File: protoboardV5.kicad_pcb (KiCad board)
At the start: 2 copper layers, 33 x 25 mm, 19 parts, among them J1 J1, J2 J2, J3 J3, M1 M1, Q1 Q1, Q2 Q2, U1 U1

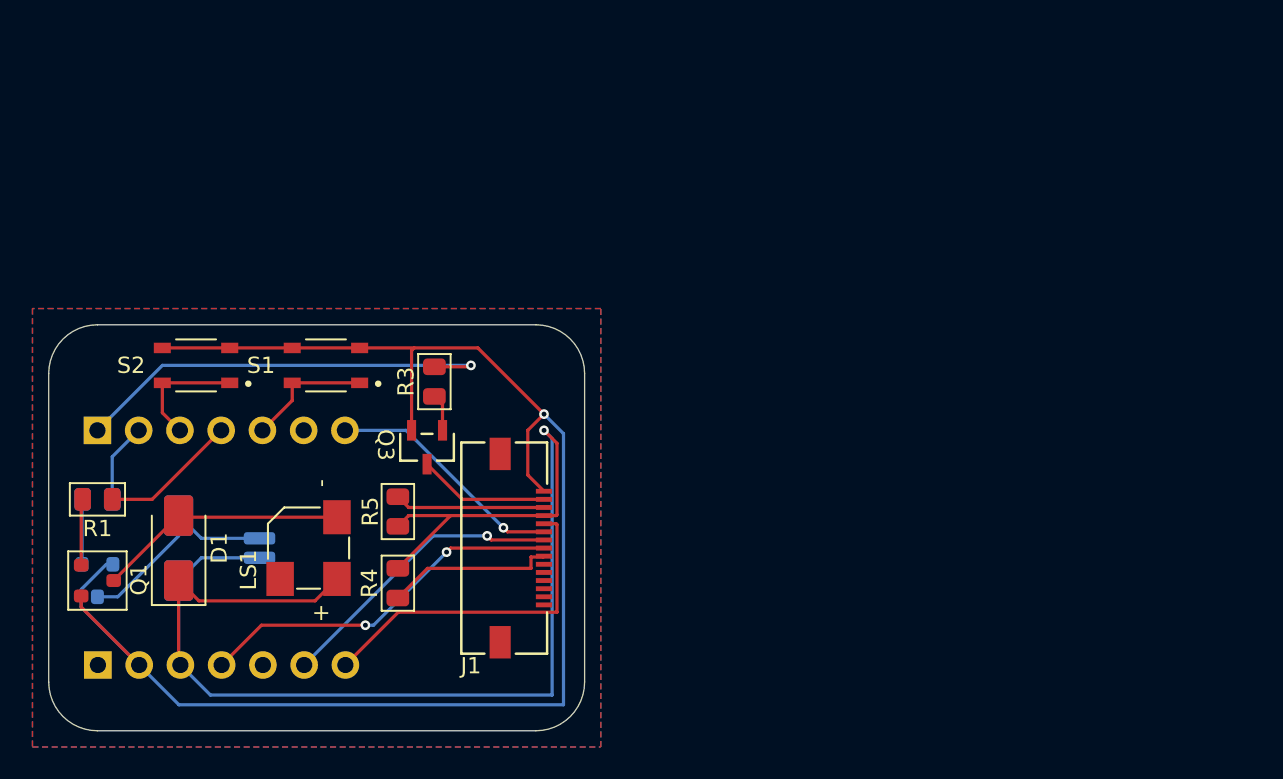
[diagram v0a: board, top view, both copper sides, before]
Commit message: Add files via upload
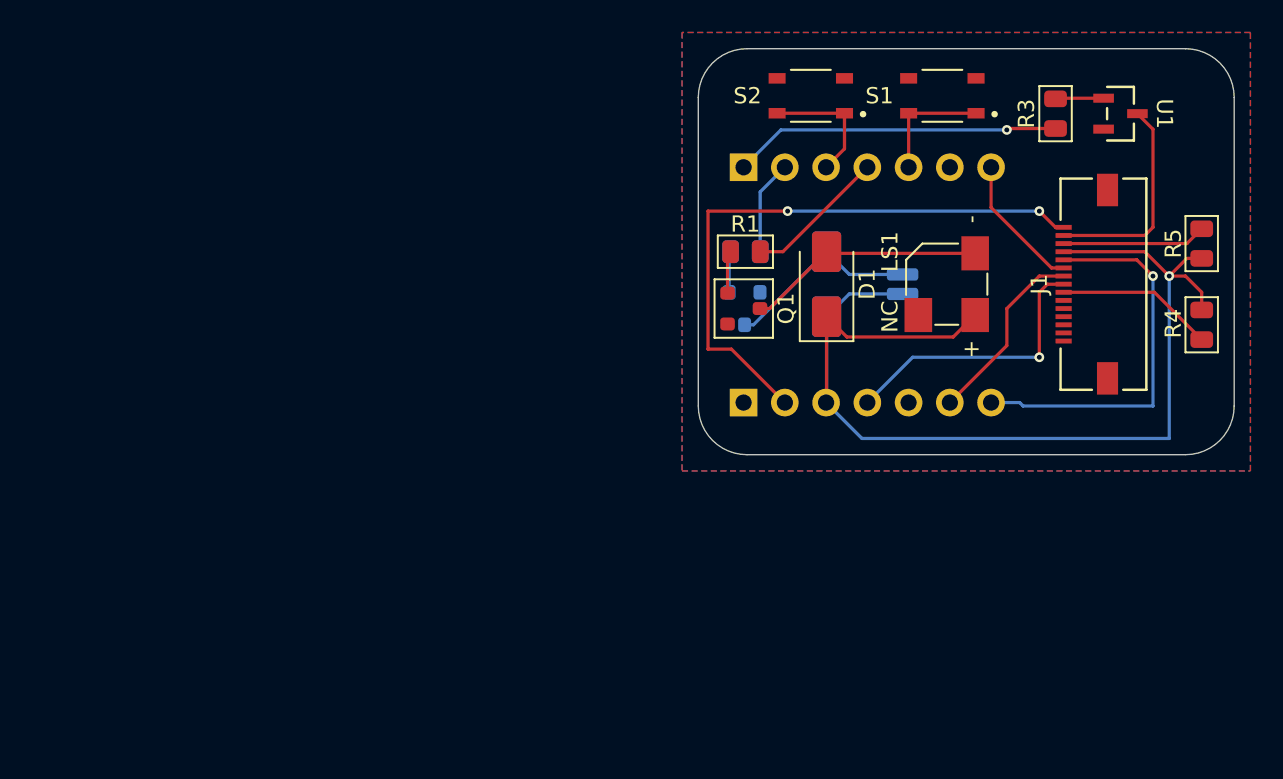
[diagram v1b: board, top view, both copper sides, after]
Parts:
- removed the G*** at (95.0, 95.0)
- removed the G*** at (95.6, 84.0)
- added G***: LOGO, LOGO, B.Cu at (135.0, 66.0)
- moved R5 52.2 mm to (140.0, 72.0)
- moved R4 52.0 mm to (140.0, 77.0)
- moved U1 47.4 mm to (135.0, 64.0), turned to -90 degrees
- moved Q2 43.2 mm to (111.8, 76.0)
- moved Q1 43.2 mm to (111.8, 76.0)
- moved D1 43.1 mm to (116.9, 74.5)
- moved D2 43.1 mm to (116.9, 74.5)
- moved J3 43.0 mm to (111.8, 67.3)
- moved J2 42.9 mm to (111.8, 81.8)
- moved M1 42.8 mm to (126.6, 74.5)
- moved R1 42.7 mm to (111.9, 72.5)
- moved R2 42.7 mm to (111.9, 72.5)
- moved LS1 42.5 mm to (124.3, 74.5)
- moved R3 41.7 mm to (131.0, 64.0), turned to 90 degrees
- moved S1 41.4 mm to (124.0, 62.9)
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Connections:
- J1 pad 1: GND -> unconnected-(J1-Pad1)
- J1 pad 10: unconnected-(J1-Pad10) -> /TX
- J1 pad 11: unconnected-(J1-Pad11) -> /RX
- J1 pad 12: unconnected-(J1-Pad12) -> +3.3V
- J1 pad 13: unconnected-(J1-Pad13) -> Net-(J1-Pad13)
- J1 pad 14: unconnected-(J1-Pad14) -> Net-(U1-D)
- J1 pad 15: unconnected-(J1-Pad15) -> GND
- J1 pad 2: Net-(U1-D) -> unconnected-(J1-Pad2)
- J1 pad 3: Net-(J1-Pad3) -> unconnected-(J1-Pad3)
- J1 pad 4: +3.3V -> unconnected-(J1-Pad4)
- J1 pad 5: /RX -> unconnected-(J1-Pad5)
- J1 pad 6: /TX -> unconnected-(J1-Pad6)
- J1 pad 7: /SCK -> Net-(J1-Pad7)
- J1 pad 9: Net-(J1-Pad9) -> /SCK
- R4 pad 2: Net-(J1-Pad9) -> Net-(J1-Pad7)
- R5 pad 2: Net-(J1-Pad3) -> Net-(J1-Pad13)
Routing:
- net GND: track 95.9 -> 37.0 mm, vias 1 -> 2
- net +3.3V: track 87.3 -> 71.2 mm
- net Net-(J1-Pad9): track 10.5 -> 0.00 mm
- net Net-(J1-Pad7): track 0.00 -> 9.71 mm
- net Net-(J1-Pad3): track 9.27 -> 0.00 mm
- net Net-(J1-Pad13): track 0.00 -> 8.88 mm
- net /A0: track 26.9 -> 20.2 mm
- net /SCK: track 18.2 -> 11.6 mm, vias 1 -> 0
- net /TX: track 14.8 -> 8.49 mm, vias 1 -> 0
- net /MOSI: track 22.8 -> 17.5 mm, vias 2 -> 1
- net Net-(U1-D): track 8.10 -> 13.1 mm
- net /RX: track 20.6 -> 24.0 mm, vias 0 -> 1
- net Net-(Q2-B): track 4.02 -> 2.54 mm
- net Net-(Q1-B): track 4.09 -> 2.63 mm
- net Net-(D2-A): track 13.4 -> 12.2 mm
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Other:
- board text removed: "Q3"
